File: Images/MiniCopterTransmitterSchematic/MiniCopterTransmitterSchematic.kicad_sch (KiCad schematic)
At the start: 4 parts

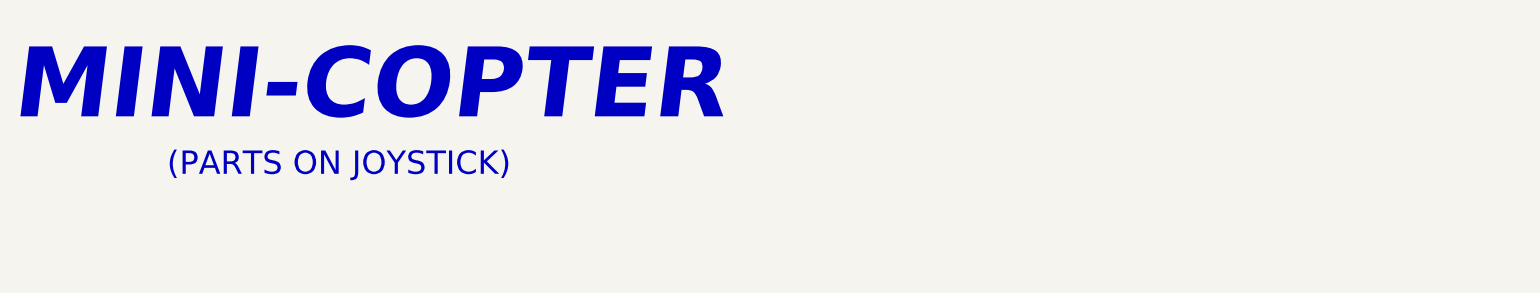
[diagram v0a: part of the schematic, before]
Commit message: Finalized PCB
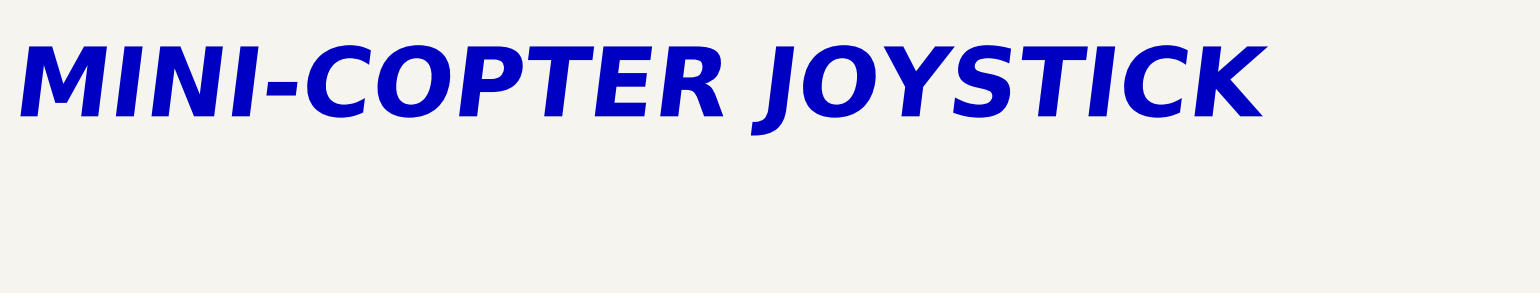
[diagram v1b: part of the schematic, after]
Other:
- note added: "MINI-COPTER JOYSTICK"
- note removed: "(PARTS ON JOYSTICK)"
- note removed: "MINI-COPTER"
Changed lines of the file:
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@@
     (stroke (width 0) (type default) (color 0 0 0 0))
   )
-  (text "(PARTS ON JOYSTICK)" (at 53.34 48.26 0)
-    (effects (font (size 4 4)) (justify left bottom))
-  )
-  (text "MINI-COPTER" (at 26.67 39.37 0)
+  (text "MINI-COPTER JOYSTICK" (at 26.67 39.37 0)
     (effects (font (size 12 12) (thickness 1.4) bold italic) (justify left bottom))
   )
